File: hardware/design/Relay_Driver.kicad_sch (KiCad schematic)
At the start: 4 parts, among them K8501 RP438012, Q8501 2N2222

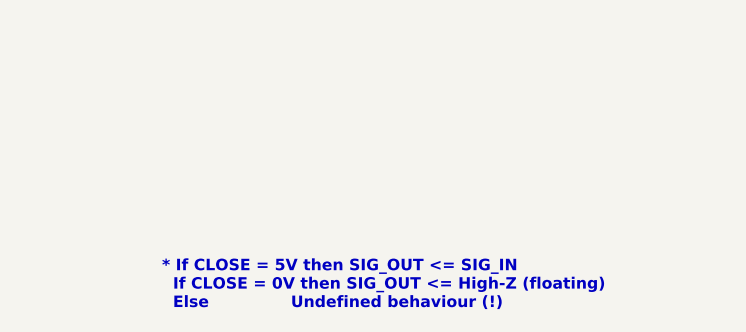
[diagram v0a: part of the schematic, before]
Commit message: File cleanup
Added final schematics
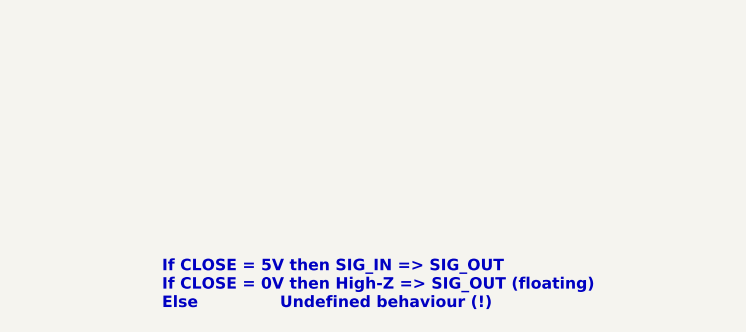
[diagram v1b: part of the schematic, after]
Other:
- note added: "If CLOSE = 5V then SIG_IN => SIG_OUT If CLOSE = 0V then High-Z => SIG_OUT (floating) Else Undefined behaviour (!)"
- note removed: "* If CLOSE = 5V then SIG_OUT <= SIG_IN If CLOSE = 0V then SIG_OUT <= High-Z (floating) Else Undefined behaviour (!)"
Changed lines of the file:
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@@
 	(title_block
 		(title "VersaLogic board tester")
-		(date "2025-08-13")
-		(rev "1.0.alpha")
+		(date "2025-09-09")
+		(rev "1.0")
 		(comment 1 "Copyright (c) 2025 by Filip Pynckels & Robin Pynckels")
 	)
@@
 		)
 	)
-	(text "* If CLOSE = 5V then SIG_OUT <= SIG_IN\n  If CLOSE = 0V then SIG_OUT <= High-Z (floating)\n  Else               Undefined behaviour (!)"
+	(text "If CLOSE = 5V then SIG_IN => SIG_OUT\nIf CLOSE = 0V then High-Z => SIG_OUT (floating)\nElse               Undefined behaviour (!)"
 		(exclude_from_sim no)
 		(at 90.424 113.03 0)
